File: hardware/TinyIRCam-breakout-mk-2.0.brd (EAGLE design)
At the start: 20 x 20 mm, 11 parts, among them J1 DF12-32-DP-NOTREALLY, U1 GRIDEYE

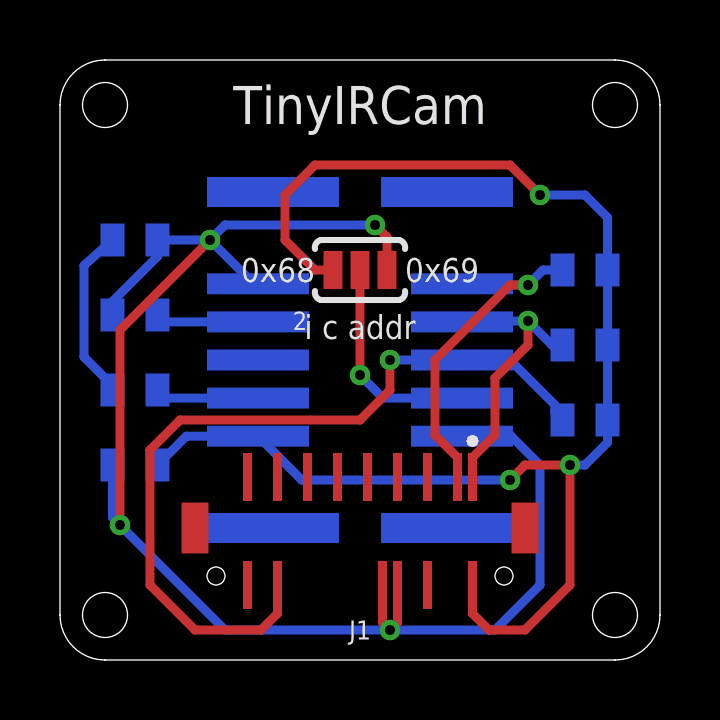
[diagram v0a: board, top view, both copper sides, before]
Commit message: whole lotta commits
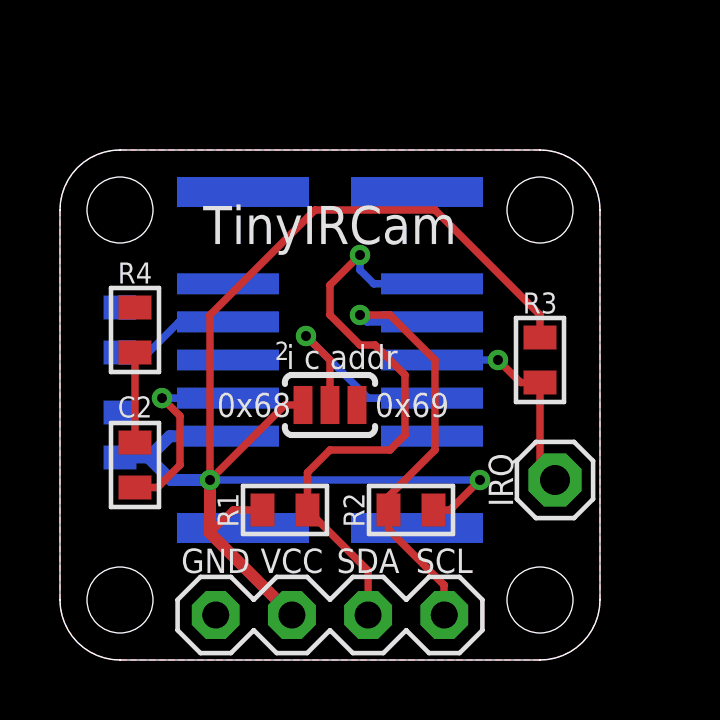
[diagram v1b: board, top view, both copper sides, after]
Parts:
- removed J1: DF12-32-DP-NOTREALLY, a_parts:DF12-32-DP-I2C+EXTRA
- added I2C: M04PTH-CENTERED, a_parts:1X04-PTH-VERT-CENTER
- added IRQ: M01PTH, a_parts:1X01
- moved R1 12.8 mm to (7.50, 5.00), flipped to the top
- moved R2 7.99 mm to (11.7, 5.00), flipped to the top, turned to 0 degrees
- moved ADDR 4.61 mm to (9.00, 8.50)
- moved R4 3.00 mm to (2.50, 11.0), flipped to the top, turned to 270 degrees
- moved C2 2.50 mm to (2.50, 6.50), flipped to the top, turned to 90 degrees
- moved R3 2.50 mm to (16.0, 10.0), flipped to the top, turned to 90 degrees
- moved C1 1.12 mm to (2.00, 7.50), turned to 90 degrees
- moved U1 1.00 mm to (9.00, 10.0)
- moved C3 0.71 mm to (2.00, 11.0), turned to 90 degrees
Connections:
- net 3.3V: now also I2C.2; no longer J1.2
- net GND: now also I2C.1; no longer J1.12, J1.14
- net INT: now also IRQ.1; no longer J1.28
- net SCL: now also I2C.4; no longer J1.1
- net SDA: now also I2C.3; no longer J1.3
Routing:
- net GND: track 53.6 -> 0.00 mm, vias 4 -> 0
- net INT: track 27.1 -> 7.37 mm
- net SDA: track 11.9 -> 20.2 mm
- net SCL: track 9.66 -> 15.5 mm
- net N$3: track 3.46 -> 6.49 mm, vias 0 -> 1
- net N$1: track 5.82 -> 3.00 mm
- net 3.3V: track 48.5 -> 49.2 mm, vias 3 -> 2
- net N$2: track 3.45 -> 4.02 mm
- added copper zone on layer 1, net GND
- added copper zone on layer 16, net GND
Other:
- board size 20 x 20 mm -> 18 x 17 mm
- board text added: "GND"
- board text added: "SCL"
- board text added: "SDA"
- board text added: "VCC"
